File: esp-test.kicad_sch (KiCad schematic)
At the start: 21 parts, among them J1 AudioPlug3, U1 ESP32-S3-WROOM-1, U2 AP2112K-3.3

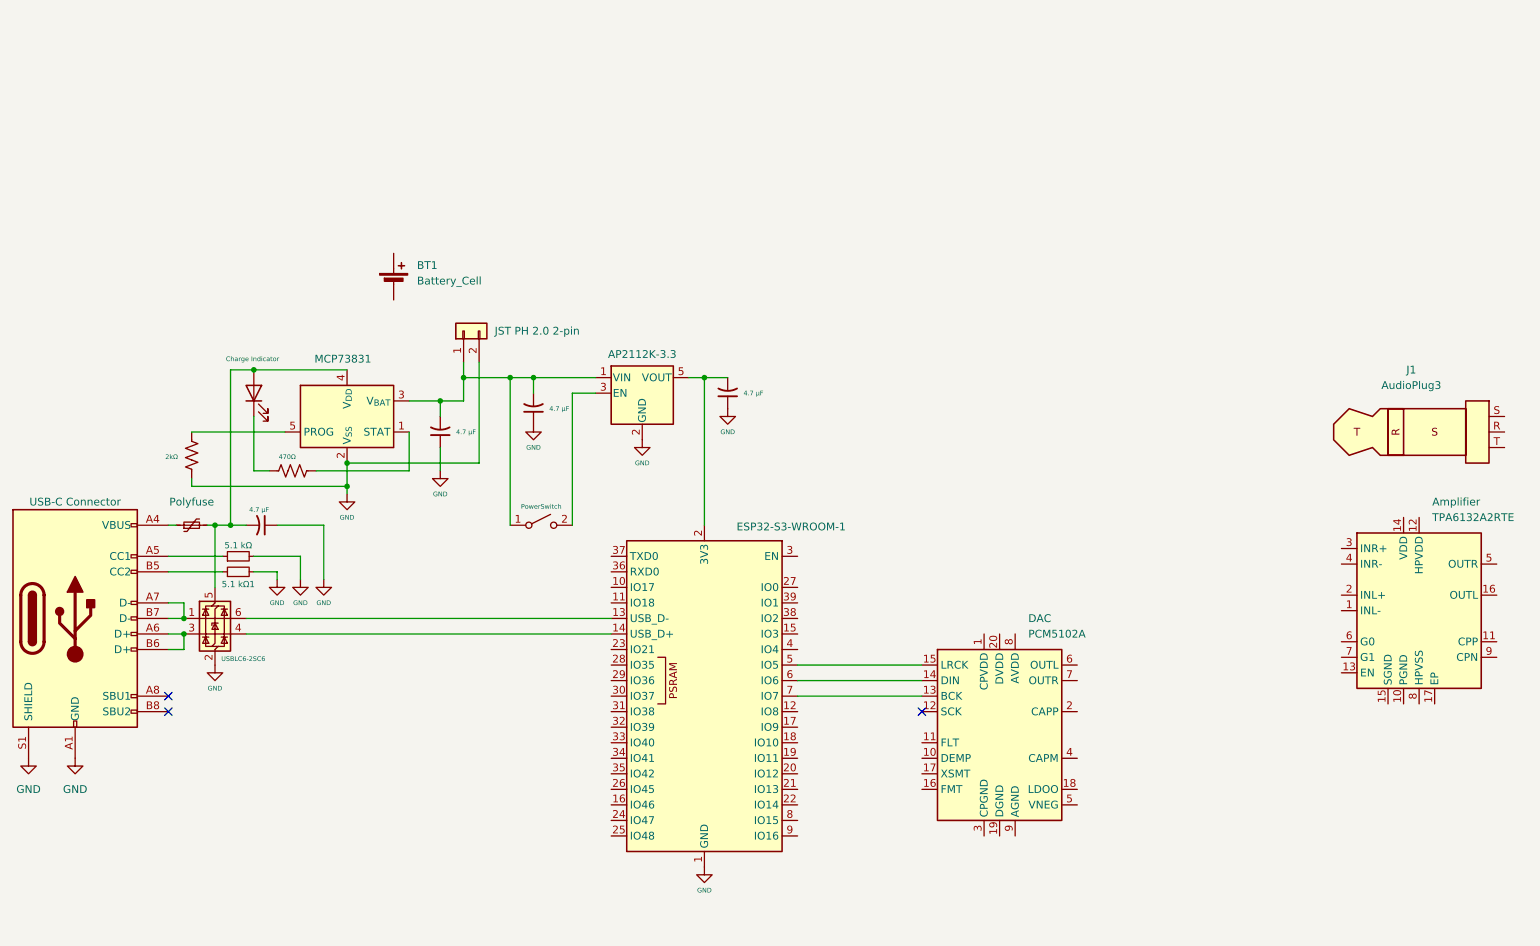
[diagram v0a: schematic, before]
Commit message: work
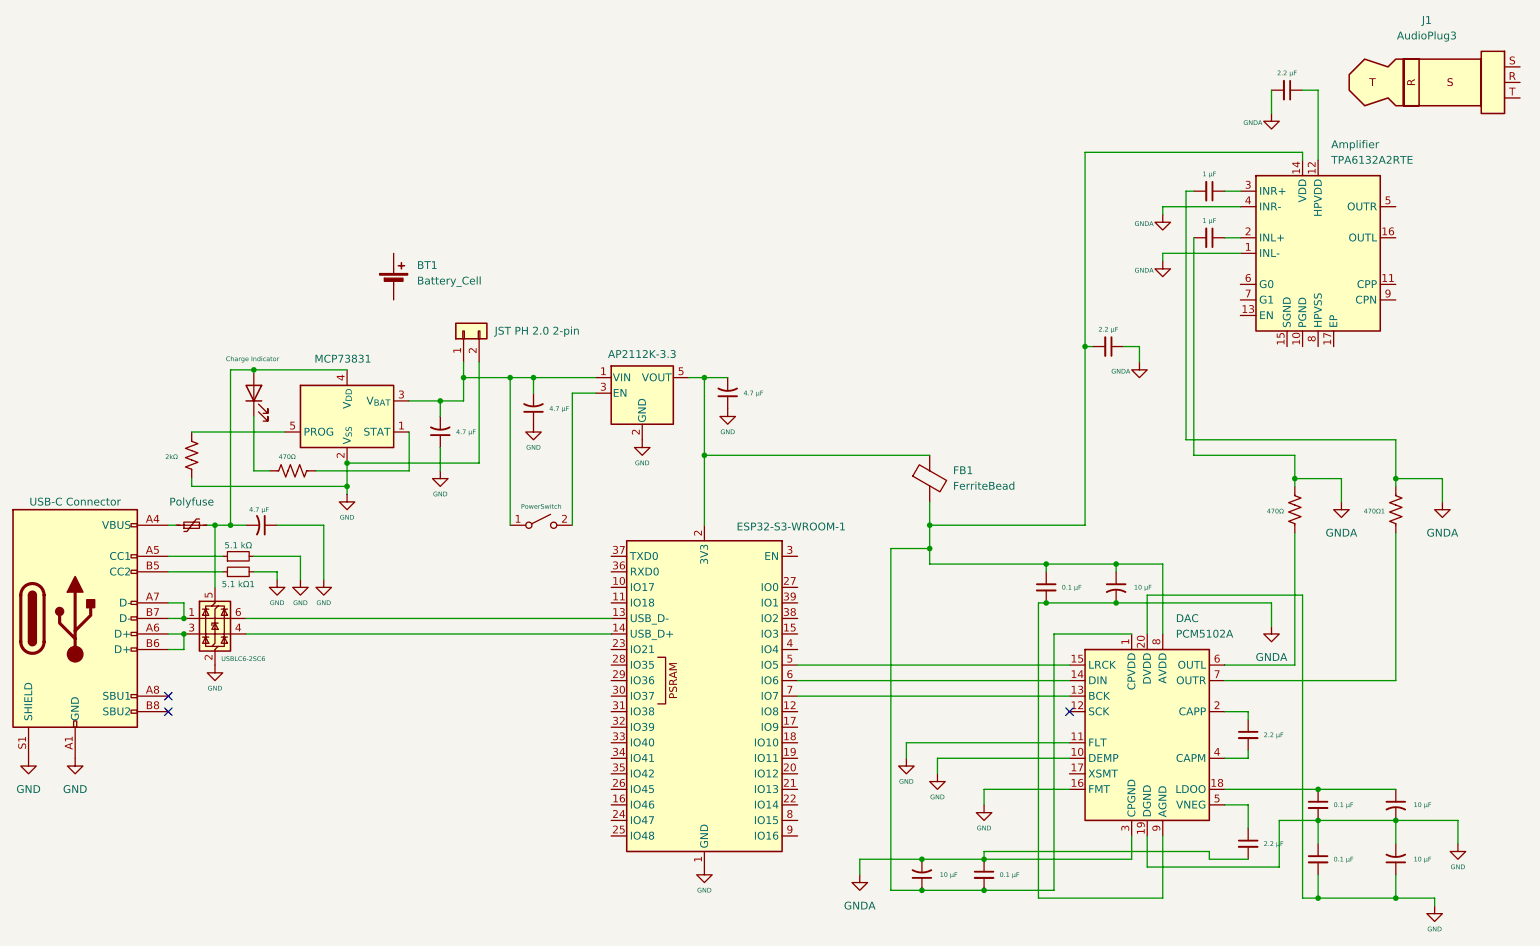
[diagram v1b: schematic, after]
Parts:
- added 470Ω, 470Ω1: R_US, symbol Device:R_US
- added C10, C14, C6, C8: 0.1 µF, symbol Device:C_Small
- added C11, C13, C5, C9: 10 µF, symbol Device:C_Small_US
- added C12, C17, C18, C7: 2.2 µF, symbol Device:C_Small
- added C15, C16: 1 µF, symbol Device:C_Small
- added FB1: FerriteBead, symbol Device:FerriteBead
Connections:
- net GND: now also DAC.10 (DEMP), DAC.11 (FLT), DAC.16 (FMT), DAC.19 (DGND), DAC.20 (DVDD), C13.1, C13.2, C14.1, C14.2, C5.2, C6.2
- net at C4.2, U1.2 (3V3), U2.5 (VOUT): now also FB1.1
- net GNDA: now reaches Amplifier.1 (INL-)
- net GNDA: now also Amplifier.4 (INR-), DAC.3 (CPGND), DAC.9 (AGND), 470Ω.2, 470Ω1.2, C10.1, C11.2, C12.2, C15.2, C16.2, C17.2, C18.1, C8.2, C9.2
- net at Amplifier.12 (HPVDD): now also C17.1
- net at Amplifier.14 (VDD): now also DAC.1 (CPVDD), DAC.8 (AVDD), C10.2, C11.1, C18.2, C8.1, C9.1, FB1.2
- net at Amplifier.2 (INL+): now also C16.1
- net at Amplifier.3 (INR+): now also C15.1
- net at DAC.18 (LDOO): now also C5.1, C6.1
- net at DAC.2 (CAPP): now also C7.1
- net at DAC.4 (CAPM): now also C7.2
- net at DAC.5 (VNEG): now also C12.1
- net at DAC.6 (OUTL): now also 470Ω.1
- net at DAC.7 (OUTR): now also 470Ω1.1
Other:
- moved on the sheet: Amplifier, DAC, J1
